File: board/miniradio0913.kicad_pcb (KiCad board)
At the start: 2 copper layers, 33 x 27.9 mm, 30 parts, among them J1 AudioJack3, J2 Conn_01x03_Socket, J3 USB_B_Micro, Q2 Q_PMOS_GSD, SW1 SW_Push, SW2 SW_Push, SW3 SW_Push, U1 CH32V003JxMx, U2 KT0913, U3 AQM0802, Y1 32.768kHz

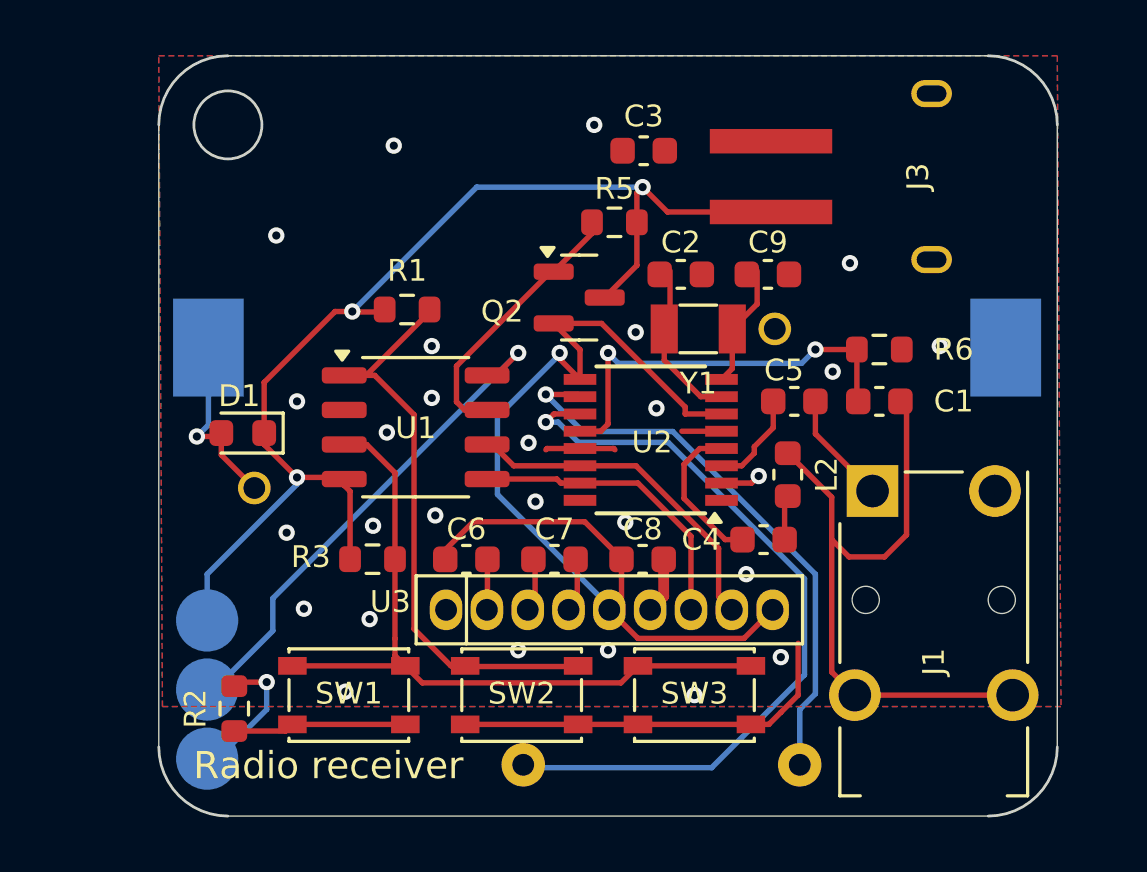
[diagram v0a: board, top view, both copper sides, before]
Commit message: board: update
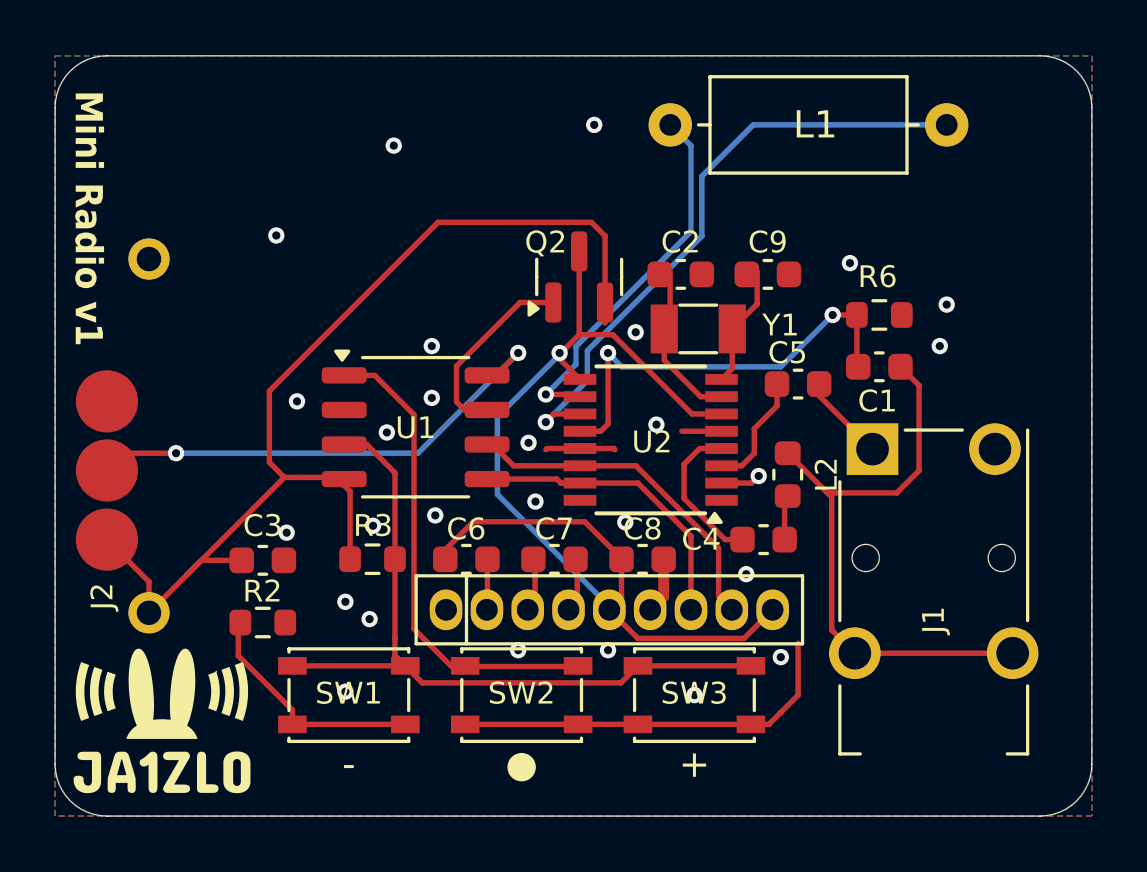
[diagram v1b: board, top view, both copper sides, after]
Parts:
- removed BT2: Battery, Library:CH25-2032LF
- removed D1: D_Small, Diode_SMD:D_0603_1608Metric
- removed J3: USB_B_Micro, Library:usb_microb_power_MRUSB-2B-D14NI-S306
- removed R1: R, Resistor_SMD:R_0603_1608Metric
- removed R5: 10k, Resistor_SMD:R_0603_1608Metric
- BT1: footprint Battery:BatteryHolder_Keystone_1060_1x2032 -> Library:BH-521_2xN
- J2, L1: moved to F.Cu
- moved L1 24.0 mm to (56.9, 19.1), turned to 0 degrees
- moved C3 20.6 mm to (41.9, 35.1)
- moved J2 8.85 mm to (36.2, 31.8), turned to 90 degrees
- moved BT1 3.47 mm to (53.3, 30.5)
- moved R2 3.33 mm to (41.9, 37.3), turned to 0 degrees
- moved J1 1.54 mm to (66.6, 37.5)
- moved C1 1.27 mm to (64.6, 27.9)
- moved R6 1.27 mm to (64.6, 26.0)
- moved Q2 0.76 mm to (53.5, 24.6), turned to 90 degrees
- moved C5 0.65 mm to (61.6, 28.6)
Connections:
- BT1 pad 1: Net-(BT1-+) -> VDD
- C6 pad 1: Net-(Q2-S) -> Net-(Q2-D)
- C8 pad 1: Net-(Q2-S) -> Net-(Q2-D)
- Q2 pad 2: Net-(Q2-S) -> VDD
- Q2 pad 3: VDD -> Net-(Q2-D)
- U2 pad 6: Net-(Q2-S) -> Net-(Q2-D)
- U2 pad 9: Net-(Q2-S) -> Net-(Q2-D)
- U3 pad 5: Net-(Q2-S) -> Net-(Q2-D)
- U3 pad 9: Net-(Q2-S) -> Net-(Q2-D)
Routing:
- net Net-(Q2-D): track 0.00 -> 40.4 mm, vias 0 -> 1
- net Net-(Q2-S): track 40.1 -> 0.00 mm, vias 1 -> 0
- net Net-(U2-AMINN): track 21.2 -> 13.7 mm
- net Net-(BT1-+): track 6.91 -> 0.00 mm, vias 1 -> 0
- net Net-(U2-AMINP): track 28.6 -> 22.6 mm
- net GND: track 27.4 -> 22.2 mm, vias 28 -> 27
- net Net-(U1-PD6/PA1): track 21.7 -> 17.6 mm
- net VDD: track 43.3 -> 39.6 mm, vias 3 -> 0
- net Net-(Q2-G): track 9.97 -> 7.09 mm
- net Net-(R2-Pad1): track 6.39 -> 8.72 mm
- net Net-(C1-Pad1): track 24.1 -> 22.0 mm
- net Net-(C5-Pad1): track 4.16 -> 3.20 mm
- net Net-(U2-ROUT): track 3.59 -> 4.28 mm
- net Net-(U2-RFINP): track 15.2 -> 15.8 mm
- net Net-(J2-Pin_2): track 18.7 -> 18.4 mm, vias 1 -> 2
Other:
- board size 33 x 27.9 mm -> 38.1 x 27.9 mm
- board text added: "+"
- board text added: "-"
- board text added: "Mini Radio v1"
- board text added: "●"
- board text removed: "Radio receiver"
